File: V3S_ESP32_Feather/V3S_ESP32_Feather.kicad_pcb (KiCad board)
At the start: 4 copper layers, 30.5 x 48.3 mm, 92 parts, among them J1 USB_B_Micro, J10 UART, J2 Bat, J3 CAM, J4 PWM, J5 U.FL-R-SMT(01), J7 Micro_SD_Card_Det, J8 I2C, J9 I2C, U1 V3S, U2 MIC5504-1.2YM5, U3 MIC5501-3.0YM5, U4 ICM-20948, U5 ESP32-PICO-D4, U6 LT1963AxST-3.3, U7 BMP280, U8 MIC5504-1.8YM5, U9 MAX13030EETE, Y1 X1E0000210832, Y2 CC5V-T1A 32.768KHZ +-20PPM 12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

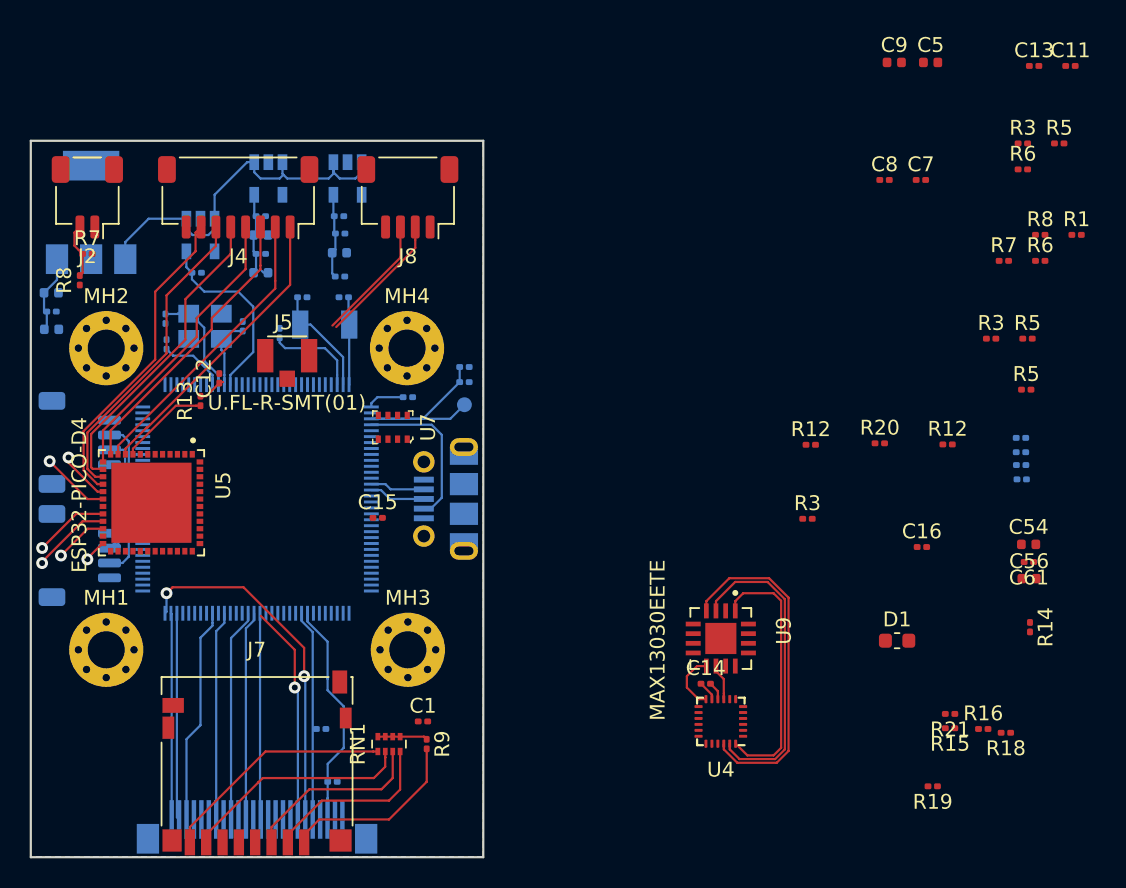
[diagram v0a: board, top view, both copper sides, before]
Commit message: ICM rooted
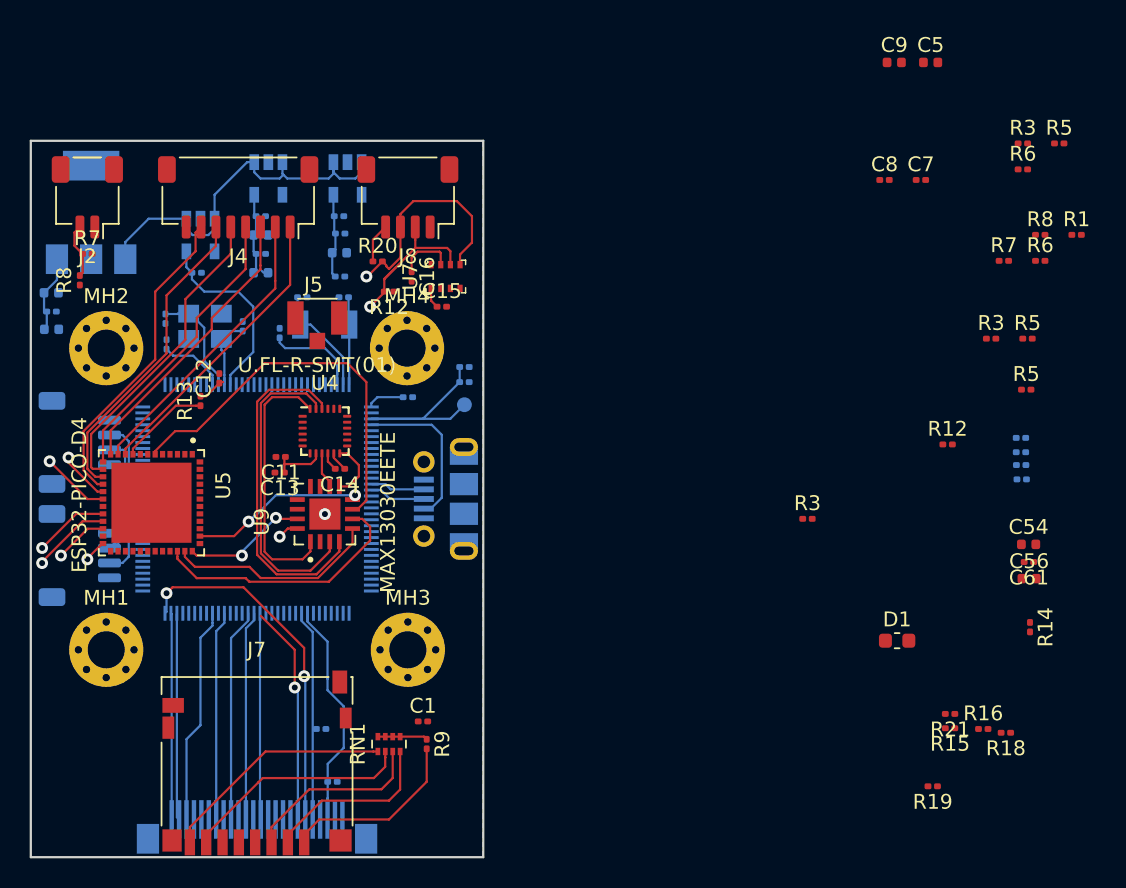
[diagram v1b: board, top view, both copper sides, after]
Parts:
- moved C11 59.4 mm to (39.7, 41.6), turned to 180 degrees
- moved C13 57.7 mm to (39.6, 42.7), turned to 180 degrees
- moved C16 38.9 mm to (48.5, 29.5), turned to 270 degrees
- moved R20 36.0 mm to (46.2, 28.4)
- moved U4 33.1 mm to (42.7, 39.9), turned to 0 degrees
- moved R12 30.2 mm to (47.0, 30.5), turned to 180 degrees
- moved C14 28.6 mm to (43.7, 42.4), turned to 180 degrees
- moved U9 28.0 mm to (42.7, 45.5), turned to 90 degrees
- moved C15 14.9 mm to (50.5, 31.5)
- moved U7 10.8 mm to (50.8, 29.5), turned to 90 degrees
- moved J5 3.25 mm to (42.2, 32.3)
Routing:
- net /WIFI, BT, RT/ICM_INT: track 0.00 -> 26.6 mm
- net /WIFI, BT, RT/CS: track 0.00 -> 17.6 mm
- net /WIFI, BT, RT/CLK: track 0.00 -> 14.2 mm
- net /WIFI, BT, RT/MISO: track 0.00 -> 12.0 mm, vias 0 -> 2
- net +3V3: track 8.78 -> 18.2 mm, vias 0 -> 1
- net /WIFI, BT, RT/MOSI: track 0.00 -> 8.42 mm, vias 0 -> 2
- net /SCL: track 8.54 -> 15.4 mm, vias 0 -> 1
- net +1V8: track 5.68 -> 9.41 mm
- net /SDA: track 8.94 -> 11.1 mm, vias 0 -> 1
- net GND: vias 0 -> 1
